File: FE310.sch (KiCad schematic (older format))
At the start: 44 parts, among them Q2 SSM3K35AMFV, Q3 SSM3K35AMFV, SW1 TACTILE_SWITCH_SMALL, SW2 TACTILE_SWITCH_SMALL, U4 FE310-G000, U5 IS25LP128-JBLE, Y1 16MHz

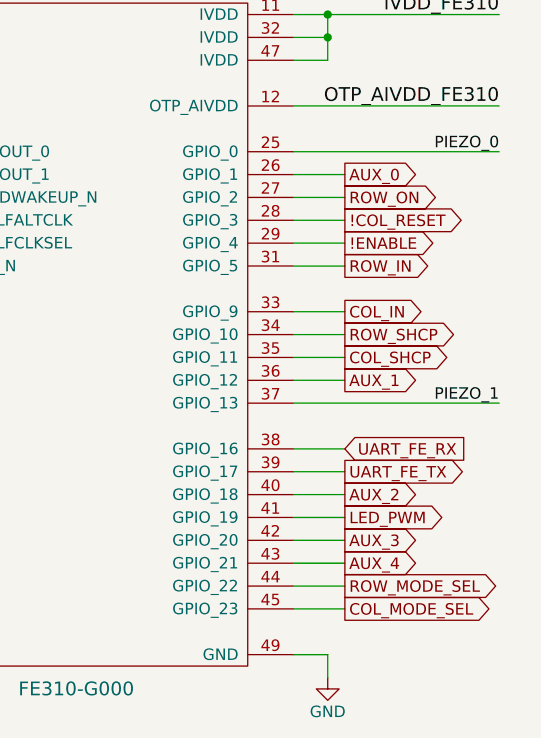
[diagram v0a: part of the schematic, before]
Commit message: automated commit
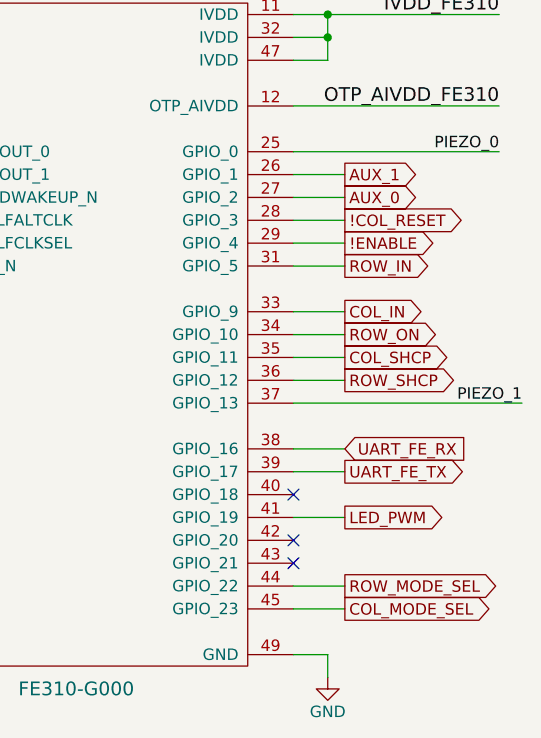
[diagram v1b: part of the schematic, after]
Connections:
- net AUX_0: now also U4.27 (GPIO_2); no longer U4.26 (GPIO_1)
- net AUX_1: now also U4.26 (GPIO_1); no longer U4.36 (GPIO_12)
- net ROW_ON: now also U4.34 (GPIO_10); no longer U4.27 (GPIO_2)
- net ROW_SHCP: now also U4.36 (GPIO_12); no longer U4.34 (GPIO_10)
- net AUX_2: no longer names the net of U4.40 (GPIO_18)
- net AUX_3: no longer names the net of U4.42 (GPIO_20)
- net AUX_4: no longer names the net of U4.43 (GPIO_21)
- no-connect marks 4 -> 7
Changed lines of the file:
@@
 	9550 5325 9325 5325
-Wire Wire Line
-	9550 5225 9325 5225
-Wire Wire Line
-	9550 5125 9325 5125
-Wire Wire Line
-	9550 4925 9325 4925
 Wire Wire Line
 	9550 5425 9325 5425
@@
 	9325 4325 9550 4325
 Wire Wire Line
-	9325 4525 10225 4525
+	9325 4525 10325 4525
 Wire Wire Line
 	9325 3425 10225 3425
@@
 	1    0    0    -1
 $EndComp
-Text GLabel 9550 3625 2    50   Output ~ 0
+Text GLabel 9550 4225 2    50   Output ~ 0
 ROW_ON
 Text GLabel 9550 3725 2    50   Output ~ 0
@@
 Text GLabel 9550 4125 2    50   Output ~ 0
 COL_IN
-Text GLabel 9550 4225 2    50   Output ~ 0
+Text GLabel 9550 4425 2    50   Output ~ 0
 ROW_SHCP
 Text GLabel 9550 4325 2    50   Output ~ 0
 COL_SHCP
-Text GLabel 9550 3525 2    50   Output ~ 0
+Text GLabel 9550 3625 2    50   Output ~ 0
 AUX_0
 Text GLabel 9550 4725 2    50   Input ~ 0
@@
 Text GLabel 9550 4825 2    50   Output ~ 0
 UART_FE_TX
-Text GLabel 9550 4425 2    50   Output ~ 0
+Text GLabel 9550 3525 2    50   Output ~ 0
 AUX_1
 Text GLabel 9550 5025 2    50   Output ~ 0
 LED_PWM
-Text GLabel 9550 4925 2    50   Output ~ 0
-AUX_2
-Text GLabel 9550 5125 2    50   Output ~ 0
-AUX_3
-Text GLabel 9550 5225 2    50   Output ~ 0
-AUX_4
 Text GLabel 9550 5325 2    50   Output ~ 0
 ROW_MODE_SEL
@@
 Text Label 10225 3425 2    50   ~ 0
 PIEZO_0
-Text Label 10225 4525 2    50   ~ 0
+Text Label 10325 4525 2    50   ~ 0
 PIEZO_1
 Text Label 6725 1800 0    50   ~ 0
@@
 Text Label 10225 2825 2    60   ~ 0
 IVDD_FE310
+NoConn ~ 9325 4925
+NoConn ~ 9325 5125
+NoConn ~ 9325 5225
 $EndSCHEMATC
